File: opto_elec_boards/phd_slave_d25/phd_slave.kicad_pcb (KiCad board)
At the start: 2 copper layers, 63 x 95.2 mm, 20 parts, among them J1 From Main Board, M4a MountingHole_4.3mm_M4, M4b MountingHole_4.3mm_M4, M4c MountingHole_4.3mm_M4, M4d MountingHole_4.3mm_M4, U1 TL082, U2 OPA551

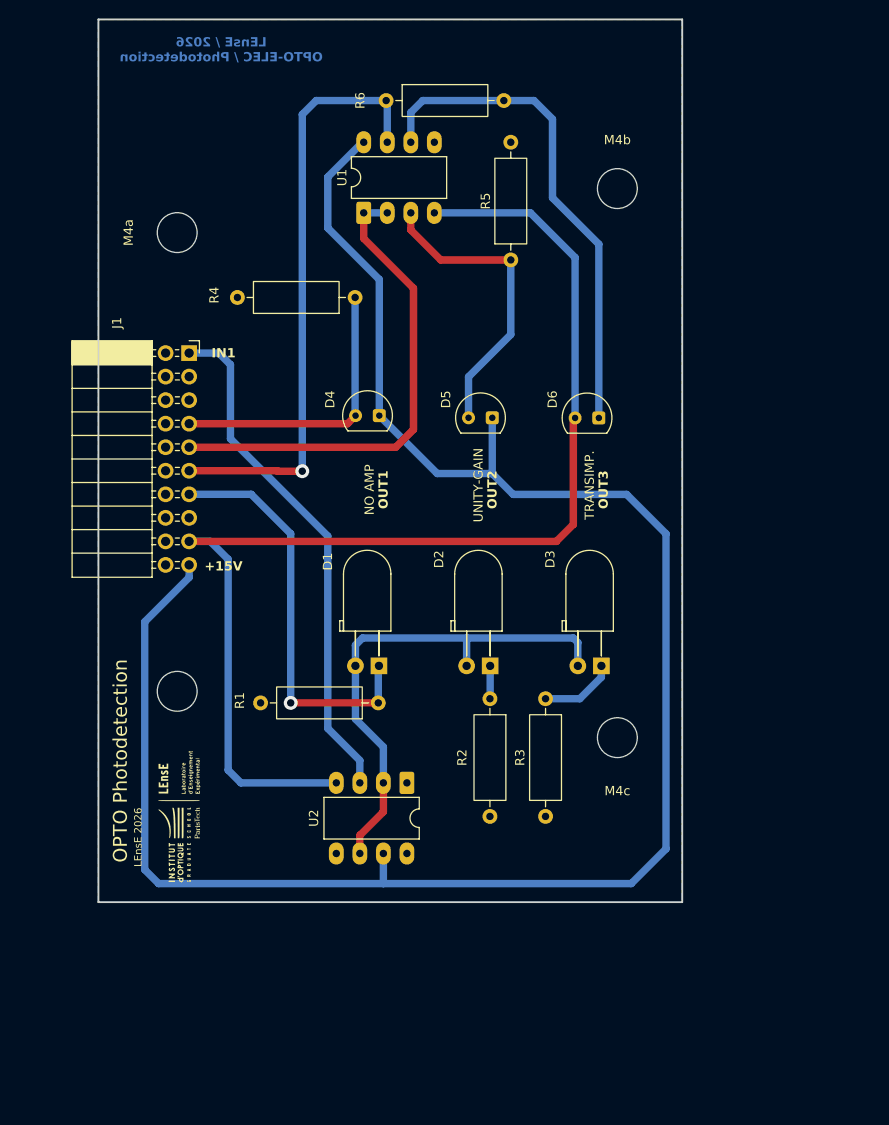
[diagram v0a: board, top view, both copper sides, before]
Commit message: Update OptoBoard / D25 version
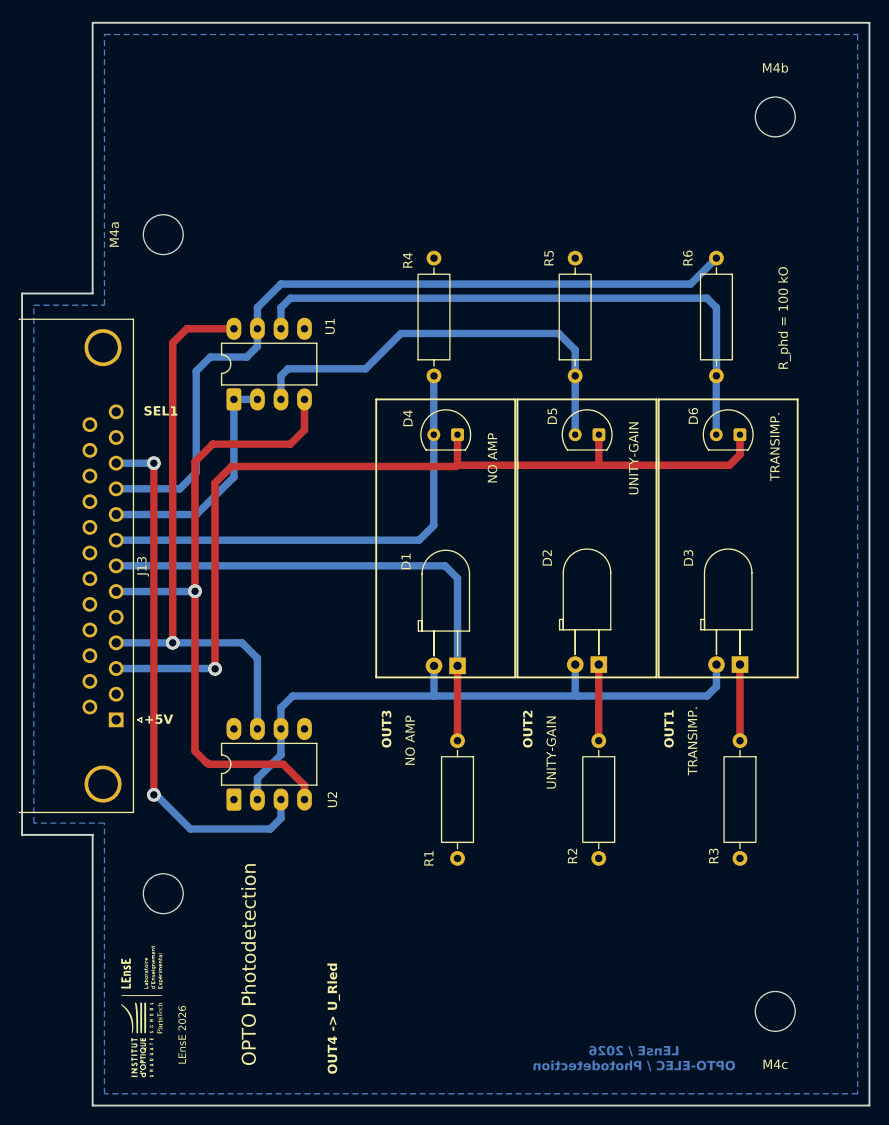
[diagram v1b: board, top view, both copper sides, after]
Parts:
- removed J1: From Main Board, Connector_PinSocket_2.54mm:PinSocket_2x10_P2.54mm_Horizontal
- added J13: FromMainBoard, Connector_Dsub:DSUB-25_Socket_Horizontal_P2.77x2.84mm_EdgePinOffset7.70mm_Housed_MountingHolesOffset9.12mm, F.Cu at (58.4, 98.1)
- moved R6 39.5 mm to (123.2, 48.3), turned to -90 degrees
- moved M4c 34.1 mm to (129.5, 129.5)
- moved U1 24.5 mm to (71.1, 63.5)
- moved M4d 21.9 mm to (63.5, 116.8)
- moved R3 21.5 mm to (125.7, 100.3)
- moved G*** 21.4 mm to (61.0, 129.5)
- moved U2 18.8 mm to (71.1, 106.7), turned to 90 degrees
- moved M4b 18.7 mm to (129.5, 33.0)
- moved D6 15.3 mm to (125.7, 67.3)
- moved D3 15.0 mm to (125.7, 92.1)
- moved R5 14.3 mm to (108.0, 61.0)
- moved R2 12.6 mm to (110.5, 100.3)
- moved R4 12.0 mm to (92.7, 61.0), turned to 90 degrees
- moved D2 11.7 mm to (110.5, 92.1)
- moved D5 11.7 mm to (110.5, 67.3)
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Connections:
- D4 pad 1: +15V -> RVAR_15V
- D4 pad 2: OUT1 -> OUT3
- D5 pad 1: +15V -> RVAR_15V
- D6 pad 1: Net-(D6-K) -> RVAR_15V
- D6 pad 2: -15V -> Net-(D6-A)
- R4 pad 1: OUT1 -> OUT3
- R6 pad 1: OUT3 -> OUT1
- R6 pad 2: Net-(D6-K) -> Net-(D6-A)
- U1 pad 6: Net-(D6-K) -> Net-(D6-A)
- U1 pad 7: OUT3 -> OUT1
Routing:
- net +15V: track 206.3 -> 63.2 mm, vias 0 -> 1
- net RVAR_15V: track 0.00 -> 97.2 mm, vias 0 -> 1
- net Net-(D6-A): track 0.00 -> 63.8 mm
- net -15V: track 128.3 -> 71.2 mm, vias 0 -> 1
- net Net-(D6-K): track 54.2 -> 0.00 mm
- net OUT1: track 31.1 -> 83.9 mm
- net OUT2: track 53.1 -> 25.3 mm
- net OUT3: track 65.0 -> 51.1 mm, vias 1 -> 0
- net LED_IN: track 54.8 -> 68.0 mm
- net Net-(D5-A): track 32.9 -> 46.1 mm
- net OUT4: track 44.5 -> 54.9 mm, vias 1 -> 0
- net Net-(D2-K): track 3.56 -> 8.22 mm
- net IN1: track 55.9 -> 57.6 mm, vias 0 -> 2
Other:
- board size 63 x 95.2 mm -> 91.4 x 116.8 mm
- board text added: "+5V"
- board text added: "OUT4 -> U_Rled"
- board text added: "R_phd = 100 kO"
- board text added: "SEL1"
- board text removed: "+15V"
- board text removed: "IN1"
